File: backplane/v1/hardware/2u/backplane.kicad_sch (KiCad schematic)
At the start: 1 part, among them J1 Conn_02x20_Odd_Even

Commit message: add board generator script & 2U backplane design
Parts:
- added H1, H11, H12, H13, H14, H15, H16, H2, H3, H4, H5, H6: MountingHole, MountingHole:MountingHole_4.3mm_M4, symbol Mechanical:MountingHole
- added H10, H17, H18, H7, H8, H9: MountingHole_Pad, MountingHole:MountingHole_3.2mm_M3_Pad, symbol Mechanical:MountingHole_Pad
- added J2, J3, J4, J5, J6, J7, J8: Conn_02x20_Odd_Even, footprints:SFM-120-X1-XXX-D, symbol Connector_Generic:Conn_02x20_Odd_Even
- J1: footprint (none) -> footprints:SFM-120-X1-XXX-D
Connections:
- net GND: now reaches J1.1 (Pin_1)
- net GND: now also J1.19 (Pin_19), J1.2 (Pin_2), J1.20 (Pin_20), J1.22 (Pin_22), J1.39 (Pin_39), J1.40 (Pin_40), J1.LC1, J1.LC2, H10.1, H17.1, H18.1, H7.1, H8.1, H9.1, J2.1 (Pin_1), J2.19 (Pin_19), J2.2 (Pin_2), J2.20 (Pin_20), J2.22 (Pin_22), J2.39 (Pin_39), J2.40 (Pin_40), J2.LC1, J2.LC2, J3.1 (Pin_1), J3.19 (Pin_19), J3.2 (Pin_2), J3.20 (Pin_20), J3.22 (Pin_22), J3.39 (Pin_39), J3.40 (Pin_40), J3.LC1, J3.LC2, J4.1 (Pin_1), J4.19 (Pin_19), J4.2 (Pin_2), J4.20 (Pin_20), J4.22 (Pin_22), J4.39 (Pin_39), J4.40 (Pin_40), J4.LC1, J4.LC2, J5.1 (Pin_1), J5.19 (Pin_19), J5.2 (Pin_2), J5.20 (Pin_20), J5.22 (Pin_22), J5.39 (Pin_39), J5.40 (Pin_40), J5.LC1, J5.LC2, J6.1 (Pin_1), J6.19 (Pin_19), J6.2 (Pin_2), J6.20 (Pin_20), J6.22 (Pin_22), J6.39 (Pin_39), J6.40 (Pin_40), J6.LC1, J6.LC2, J7.1 (Pin_1), J7.19 (Pin_19), J7.2 (Pin_2), J7.20 (Pin_20), J7.22 (Pin_22), J7.39 (Pin_39), J7.40 (Pin_40), J7.LC1, J7.LC2, J8.1 (Pin_1), J8.19 (Pin_19), J8.2 (Pin_2), J8.20 (Pin_20), J8.22 (Pin_22), J8.39 (Pin_39), J8.40 (Pin_40), J8.LC1, J8.LC2
- net RAIL_4_VOUT: now reaches J1.10 (Pin_10)
- net RAIL_4_VOUT: now also J1.9 (Pin_9), J2.10 (Pin_10), J2.9 (Pin_9), J3.10 (Pin_10), J3.9 (Pin_9), J4.10 (Pin_10), J4.9 (Pin_9), J5.10 (Pin_10), J5.9 (Pin_9), J6.10 (Pin_10), J6.9 (Pin_9), J7.10 (Pin_10), J7.9 (Pin_9), J8.10 (Pin_10), J8.9 (Pin_9)
- net RAIL_5_VOUT: now reaches J1.11 (Pin_11)
- net RAIL_5_VOUT: now also J1.12 (Pin_12), J2.11 (Pin_11), J2.12 (Pin_12), J3.11 (Pin_11), J3.12 (Pin_12), J4.11 (Pin_11), J4.12 (Pin_12), J5.11 (Pin_11), J5.12 (Pin_12), J6.11 (Pin_11), J6.12 (Pin_12), J7.11 (Pin_11), J7.12 (Pin_12), J8.11 (Pin_11), J8.12 (Pin_12)
- net RAIL_6_VOUT: now reaches J1.13 (Pin_13)
- net RAIL_6_VOUT: now also J1.14 (Pin_14), J2.13 (Pin_13), J2.14 (Pin_14), J3.13 (Pin_13), J3.14 (Pin_14), J4.13 (Pin_13), J4.14 (Pin_14), J5.13 (Pin_13), J5.14 (Pin_14), J6.13 (Pin_13), J6.14 (Pin_14), J7.13 (Pin_13), J7.14 (Pin_14), J8.13 (Pin_13), J8.14 (Pin_14)
- net RAIL_7_VOUT: now reaches J1.15 (Pin_15)
- net RAIL_7_VOUT: now also J1.16 (Pin_16), J2.15 (Pin_15), J2.16 (Pin_16), J3.15 (Pin_15), J3.16 (Pin_16), J4.15 (Pin_15), J4.16 (Pin_16), J5.15 (Pin_15), J5.16 (Pin_16), J6.15 (Pin_15), J6.16 (Pin_16), J7.15 (Pin_15), J7.16 (Pin_16), J8.15 (Pin_15), J8.16 (Pin_16)
- net RAIL_8_VOUT: now reaches J1.17 (Pin_17)
- net RAIL_8_VOUT: now also J1.18 (Pin_18), J2.17 (Pin_17), J2.18 (Pin_18), J3.17 (Pin_17), J3.18 (Pin_18), J4.17 (Pin_17), J4.18 (Pin_18), J5.17 (Pin_17), J5.18 (Pin_18), J6.17 (Pin_17), J6.18 (Pin_18), J7.17 (Pin_17), J7.18 (Pin_18), J8.17 (Pin_17), J8.18 (Pin_18)
- net EPS_PGOOD: now reaches J1.21 (Pin_21)
- net EPS_PGOOD: now also J2.21 (Pin_21), J3.21 (Pin_21), J4.21 (Pin_21), J5.21 (Pin_21), J6.21 (Pin_21), J7.21 (Pin_21), J8.21 (Pin_21)
- net CAN_MAIN_P: now reaches J1.23 (Pin_23)
- net CAN_MAIN_P: now also J1.24 (Pin_24), J2.23 (Pin_23), J2.24 (Pin_24), J3.23 (Pin_23), J3.24 (Pin_24), J4.23 (Pin_23), J4.24 (Pin_24), J5.23 (Pin_23), J5.24 (Pin_24), J6.23 (Pin_23), J6.24 (Pin_24), J7.23 (Pin_23), J7.24 (Pin_24), J8.23 (Pin_23), J8.24 (Pin_24)
- net CAN_MAIN_N: now reaches J1.25 (Pin_25)
- net CAN_MAIN_N: now also J1.26 (Pin_26), J2.25 (Pin_25), J2.26 (Pin_26), J3.25 (Pin_25), J3.26 (Pin_26), J4.25 (Pin_25), J4.26 (Pin_26), J5.25 (Pin_25), J5.26 (Pin_26), J6.25 (Pin_25), J6.26 (Pin_26), J7.25 (Pin_25), J7.26 (Pin_26), J8.25 (Pin_25), J8.26 (Pin_26)
- net OBC_HEARTBEAT: now reaches J1.27 (Pin_27)
- net OBC_HEARTBEAT: now also J2.27 (Pin_27), J3.27 (Pin_27), J4.27 (Pin_27), J5.27 (Pin_27), J6.27 (Pin_27), J7.27 (Pin_27), J8.27 (Pin_27)
- net EPS_OBC_RESET: now reaches J1.28 (Pin_28)
- net EPS_OBC_RESET: now also J2.28 (Pin_28), J3.28 (Pin_28), J4.28 (Pin_28), J5.28 (Pin_28), J6.28 (Pin_28), J7.28 (Pin_28), J8.28 (Pin_28)
- net SLOT_ID0: now reaches J1.29 (Pin_29)
- net SLOT_ID0: now also J2.29 (Pin_29), J3.29 (Pin_29), J4.29 (Pin_29), J5.29 (Pin_29), J6.29 (Pin_29), J7.29 (Pin_29), J8.29 (Pin_29)
- net RAIL_1_VOUT: now reaches J1.3 (Pin_3)
- net RAIL_1_VOUT: now also J1.4 (Pin_4), J2.3 (Pin_3), J2.4 (Pin_4), J3.3 (Pin_3), J3.4 (Pin_4), J4.3 (Pin_3), J4.4 (Pin_4), J5.3 (Pin_3), J5.4 (Pin_4), J6.3 (Pin_3), J6.4 (Pin_4), J7.3 (Pin_3), J7.4 (Pin_4), J8.3 (Pin_3), J8.4 (Pin_4)
- net OBC_EPS_RESET: now reaches J1.30 (Pin_30)
- net OBC_EPS_RESET: now also J2.30 (Pin_30), J3.30 (Pin_30), J4.30 (Pin_30), J5.30 (Pin_30), J6.30 (Pin_30), J7.30 (Pin_30), J8.30 (Pin_30)
- net SLOT_ID1: now reaches J1.31 (Pin_31)
- net SLOT_ID1: now also J2.31 (Pin_31), J3.31 (Pin_31), J4.31 (Pin_31), J5.31 (Pin_31), J6.31 (Pin_31), J7.31 (Pin_31), J8.31 (Pin_31)
- net SLOT_ID2: now reaches J1.32 (Pin_32)
- net SLOT_ID2: now also J2.32 (Pin_32), J3.32 (Pin_32), J4.32 (Pin_32), J5.32 (Pin_32), J6.32 (Pin_32), J7.32 (Pin_32), J8.32 (Pin_32)
- net SPI_SCLK: now reaches J1.33 (Pin_33)
- net SPI_SCLK: now also J2.33 (Pin_33), J3.33 (Pin_33), J4.33 (Pin_33), J5.33 (Pin_33), J6.33 (Pin_33), J7.33 (Pin_33), J8.33 (Pin_33)
- net SPI_MOSI: now reaches J1.34 (Pin_34)
- net SPI_MOSI: now also J2.34 (Pin_34), J3.34 (Pin_34), J4.34 (Pin_34), J5.34 (Pin_34), J6.34 (Pin_34), J7.34 (Pin_34), J8.34 (Pin_34)
- net SPI_MISO: now reaches J1.35 (Pin_35)
- net SPI_MISO: now also J2.35 (Pin_35), J3.35 (Pin_35), J4.35 (Pin_35), J5.35 (Pin_35), J6.35 (Pin_35), J7.35 (Pin_35), J8.35 (Pin_35)
- net CAN_AUX_P: now reaches J1.36 (Pin_36)
- net CAN_AUX_P: now also J2.36 (Pin_36), J3.36 (Pin_36), J4.36 (Pin_36), J5.36 (Pin_36), J6.36 (Pin_36), J7.36 (Pin_36), J8.36 (Pin_36)
- net SPARE1: now reaches J1.37 (Pin_37)
- net SPARE1: now also J2.37 (Pin_37), J3.37 (Pin_37), J4.37 (Pin_37), J5.37 (Pin_37), J6.37 (Pin_37), J7.37 (Pin_37), J8.37 (Pin_37)
- net CAN_AUX_N: now reaches J1.38 (Pin_38)
- net CAN_AUX_N: now also J2.38 (Pin_38), J3.38 (Pin_38), J4.38 (Pin_38), J5.38 (Pin_38), J6.38 (Pin_38), J7.38 (Pin_38), J8.38 (Pin_38)
- net RAIL_2_VOUT: now reaches J1.5 (Pin_5)
- net RAIL_2_VOUT: now also J1.6 (Pin_6), J2.5 (Pin_5), J2.6 (Pin_6), J3.5 (Pin_5), J3.6 (Pin_6), J4.5 (Pin_5), J4.6 (Pin_6), J5.5 (Pin_5), J5.6 (Pin_6), J6.5 (Pin_5), J6.6 (Pin_6), J7.5 (Pin_5), J7.6 (Pin_6), J8.5 (Pin_5), J8.6 (Pin_6)
- net RAIL_3_VOUT: now reaches J1.7 (Pin_7)
- net RAIL_3_VOUT: now also J1.8 (Pin_8), J2.7 (Pin_7), J2.8 (Pin_8), J3.7 (Pin_7), J3.8 (Pin_8), J4.7 (Pin_7), J4.8 (Pin_8), J5.7 (Pin_7), J5.8 (Pin_8), J6.7 (Pin_7), J6.8 (Pin_8), J7.7 (Pin_7), J7.8 (Pin_8), J8.7 (Pin_7), J8.8 (Pin_8)
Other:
- note added: "ADCS"
- note added: "BAT"
- note added: "COMM"
- note added: "EPS"
- note added: "GENERIC"
- note added: "OBC"
- note added: "PAYLOAD"
- note added: "Recommended Stackup: JLC04161H-7628"

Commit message: reconfigure slot ID on 2u and fix DRC
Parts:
- J1, J2, J3, J4, J5, J6, J7, J8: footprint footprints:SFM-120-X1-XXX-D -> OSUSAT_Connectors:SFM-120-X1-XXX-D
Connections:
- net GND: now also J1.32 (Pin_32), J2.29 (Pin_29), J2.32 (Pin_32), J3.29 (Pin_29), J3.31 (Pin_31), J3.32 (Pin_32), J4.31 (Pin_31), J4.32 (Pin_32), J5.29 (Pin_29), J5.31 (Pin_31), J6.31 (Pin_31), J7.29 (Pin_29)
- removed net SLOT_ID0: J1.29 (Pin_29), J2.29 (Pin_29), J3.29 (Pin_29), J4.29 (Pin_29), J5.29 (Pin_29), J6.29 (Pin_29), J7.29 (Pin_29), J8.29 (Pin_29)
- removed net SLOT_ID1: J1.31 (Pin_31), J2.31 (Pin_31), J3.31 (Pin_31), J4.31 (Pin_31), J5.31 (Pin_31), J6.31 (Pin_31), J7.31 (Pin_31), J8.31 (Pin_31)
- removed net SLOT_ID2: J1.32 (Pin_32), J2.32 (Pin_32), J3.32 (Pin_32), J4.32 (Pin_32), J5.32 (Pin_32), J6.32 (Pin_32), J7.32 (Pin_32), J8.32 (Pin_32)
- no-connect marks 0 -> 12
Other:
- moved on the sheet: H17, H18

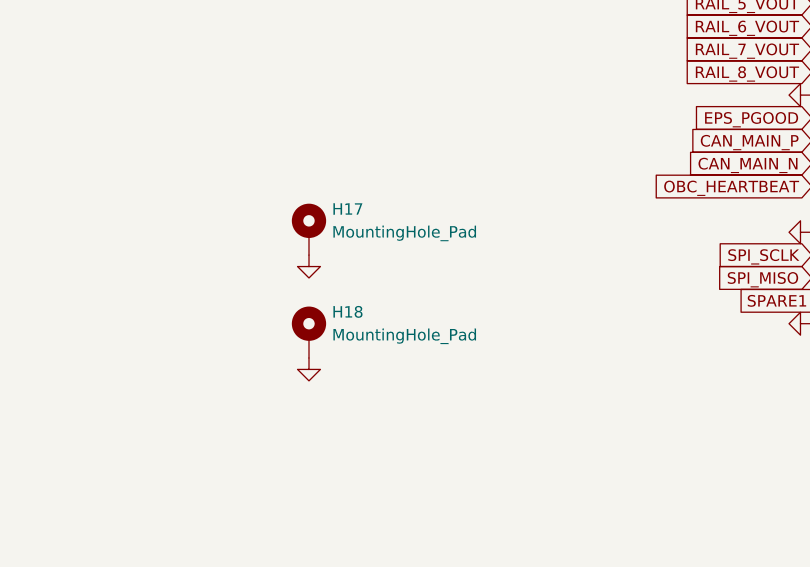
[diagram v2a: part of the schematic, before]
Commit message: fix mechanical constraints
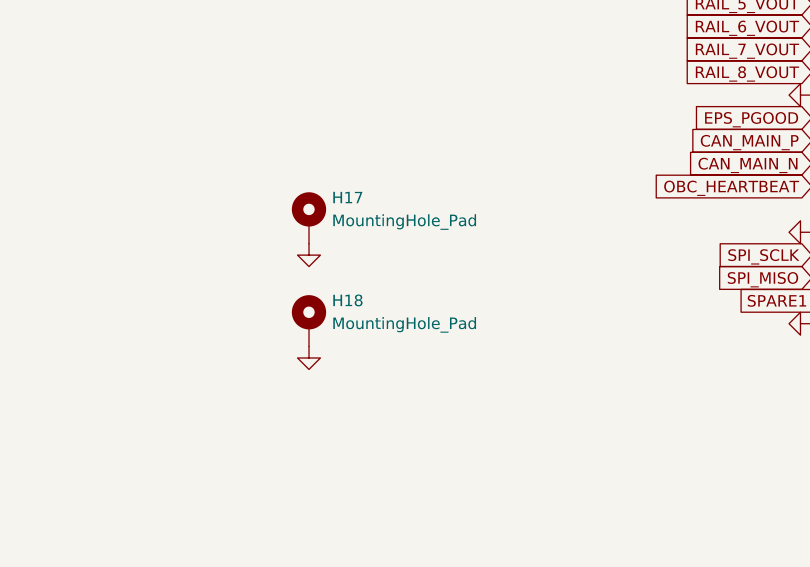
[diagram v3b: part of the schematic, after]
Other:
- moved on the sheet: H17, H18
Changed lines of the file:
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@@
 	(symbol
 		(lib_id "Mechanical:MountingHole_Pad")
-		(at 311.15 149.86 0)
+		(at 311.15 148.59 0)
 		(unit 1)
 		(body_style 1)
@@
 		(fields_autoplaced yes)
 		(property "Reference" "H17"
-			(at 313.69 147.3199 0)
+			(at 313.69 146.0499 0)
 			(show_name no)
 			(do_not_autoplace no)
@@
 		)
 		(property "Value" "MountingHole_Pad"
-			(at 313.69 149.8599 0)
+			(at 313.69 148.5899 0)
 			(show_name no)
 			(do_not_autoplace no)
@@
 		)
 		(property "Footprint" "MountingHole:MountingHole_3.2mm_M3_Pad"
-			(at 311.15 149.86 0)
+			(at 311.15 148.59 0)
 			(hide yes)
 			(show_name no)
@@
 		)
 		(property "Datasheet" ""
-			(at 311.15 149.86 0)
+			(at 311.15 148.59 0)
 			(hide yes)
 			(show_name no)
@@
 		)
 		(property "Description" "Mounting Hole with connection"
-			(at 311.15 149.86 0)
+			(at 311.15 148.59 0)
 			(hide yes)
 			(show_name no)
@@
 	(symbol
 		(lib_id "power:GND")
-		(at 311.15 163.83 0)
+		(at 311.15 162.56 0)
 		(unit 1)
 		(body_style 1)
@@
 		(fields_autoplaced yes)
 		(property "Reference" "#PWR070"
-			(at 311.15 170.18 0)
+			(at 311.15 168.91 0)
 			(hide yes)
 			(show_name no)
@@
 		)
 		(property "Value" "GND"
-			(at 311.15 168.91 0)
+			(at 311.15 167.64 0)
 			(hide yes)
 			(show_name no)
@@
 		)
 		(property "Footprint" ""
-			(at 311.15 163.83 0)
+			(at 311.15 162.56 0)
 			(hide yes)
 			(show_name no)
@@
 		)
 		(property "Datasheet" ""
-			(at 311.15 163.83 0)
+			(at 311.15 162.56 0)
 			(hide yes)
 			(show_name no)
@@
 		)
 		(property "Description" "Power symbol creates a global label with name \"GND\" , ground"
-			(at 311.15 163.83 0)
+			(at 311.15 162.56 0)
 			(hide yes)
 			(show_name no)
@@
 	(symbol
 		(lib_id "Mechanical:MountingHole_Pad")
-		(at 311.15 161.29 0)
+		(at 311.15 160.02 0)
 		(unit 1)
 		(body_style 1)
@@
 		(fields_autoplaced yes)
 		(property "Reference" "H18"
-			(at 313.69 158.7499 0)
+			(at 313.69 157.4799 0)
 			(show_name no)
 			(do_not_autoplace no)
@@
 		)
 		(property "Value" "MountingHole_Pad"
-			(at 313.69 161.2899 0)
+			(at 313.69 160.0199 0)
 			(show_name no)
 			(do_not_autoplace no)
@@
 		)
 		(property "Footprint" "MountingHole:MountingHole_3.2mm_M3_Pad"
-			(at 311.15 161.29 0)
+			(at 311.15 160.02 0)
 			(hide yes)
 			(show_name no)
@@
 		)
 		(property "Datasheet" ""
-			(at 311.15 161.29 0)
+			(at 311.15 160.02 0)
 			(hide yes)
 			(show_name no)
@@
 		)
 		(property "Description" "Mounting Hole with connection"
-			(at 311.15 161.29 0)
+			(at 311.15 160.02 0)
 			(hide yes)
 			(show_name no)
@@
 	(symbol
 		(lib_id "power:GND")
-		(at 311.15 152.4 0)
+		(at 311.15 151.13 0)
 		(unit 1)
 		(body_style 1)
@@
 		(fields_autoplaced yes)
 		(property "Reference" "#PWR069"
-			(at 311.15 158.75 0)
+			(at 311.15 157.48 0)
 			(hide yes)
 			(show_name no)
@@
 		)
 		(property "Value" "GND"
-			(at 311.15 157.48 0)
+			(at 311.15 156.21 0)
 			(hide yes)
 			(show_name no)
@@
 		)
 		(property "Footprint" ""
-			(at 311.15 152.4 0)
+			(at 311.15 151.13 0)
 			(hide yes)
 			(show_name no)
@@
 		)
 		(property "Datasheet" ""
-			(at 311.15 152.4 0)
+			(at 311.15 151.13 0)
 			(hide yes)
 			(show_name no)
@@
 		)
 		(property "Description" "Power symbol creates a global label with name \"GND\" , ground"
-			(at 311.15 152.4 0)
+			(at 311.15 151.13 0)
 			(hide yes)
 			(show_name no)
